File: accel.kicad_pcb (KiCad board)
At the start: 2 copper layers, 33 x 58 mm, 3 parts, among them U1 CH376T, U2 MPU-6050

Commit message: updates
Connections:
- A1 pad 7: unconnected-(A1-Pad7) -> Net-(A1-Pad7)
- U1 pad 13: unconnected-(U1-Pad13) -> Net-(A1-Pad7)

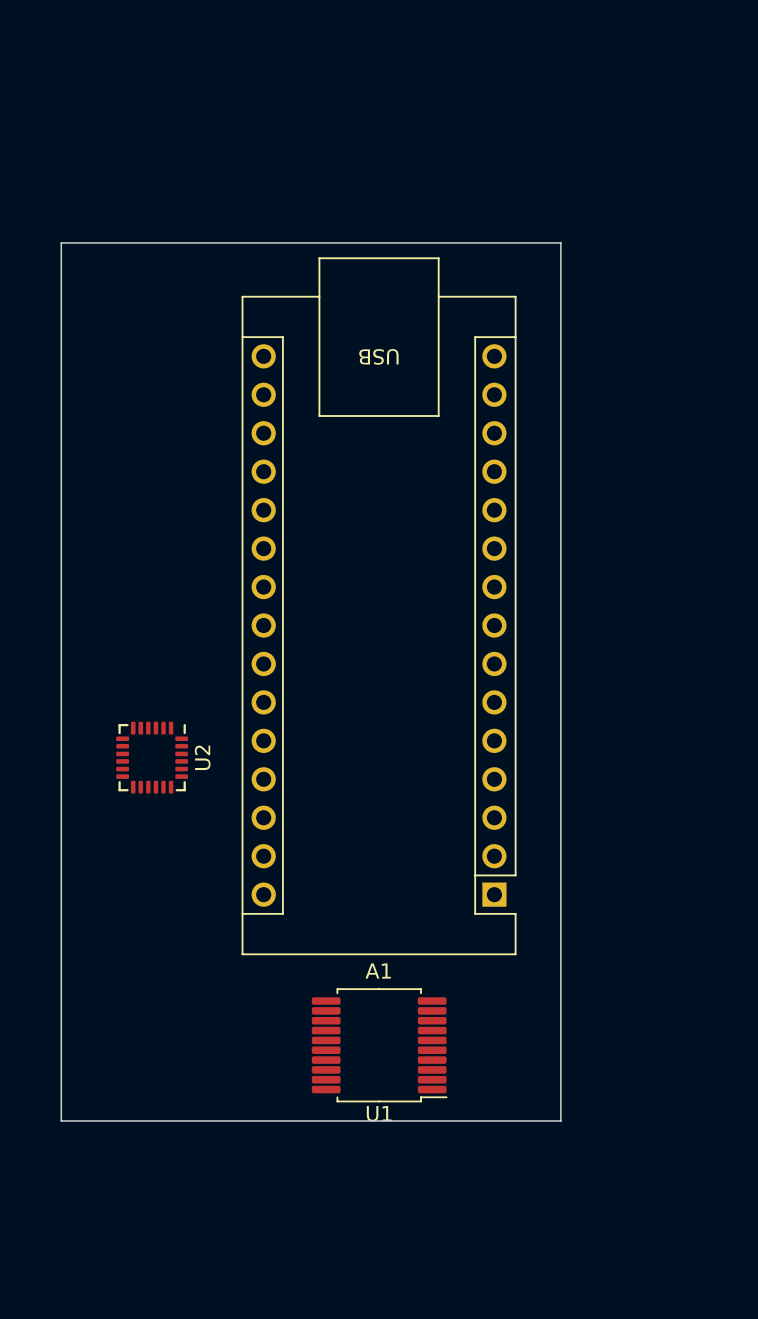
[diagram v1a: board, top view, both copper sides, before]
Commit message: final .ino and cad updates
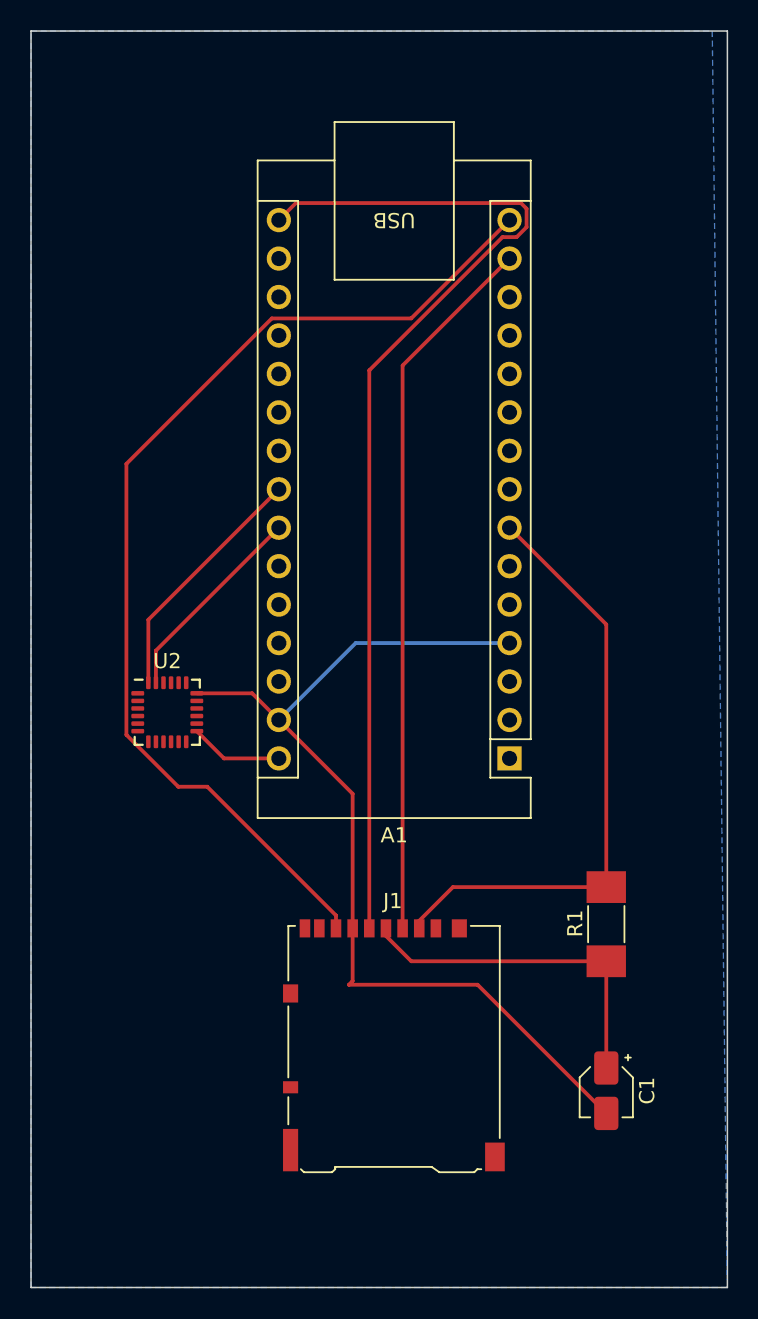
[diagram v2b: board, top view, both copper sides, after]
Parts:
- removed U1: CH376T, Package_SO:SSOP-20_5.3x7.2mm_P0.65mm
- added C1: 100nF, Capacitor_SMD:CP_Elec_3x5.4, F.Cu at (169.0, 131.0)
- added J1: Micro_SD_Card, Connector_Card:microSD_HC_Hirose_DM3AT-SF-PEJM5, F.Cu at (155.0, 128.0)
- added R1: 1K, Resistor_SMD:R_MELF_MMB-0207, F.Cu at (169.0, 120.0)
- moved A1 9.06 mm to (162.6, 109.0)
- moved U2 3.16 mm to (140.0, 106.0), turned to 0 degrees
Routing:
- net Net-(A1-Pad15): track 0.00 -> 69.5 mm
- net Net-(A1-Pad16): track 0.00 -> 69.4 mm
- net GND: track 0.00 -> 63.6 mm
- net Net-(A1-Pad14): track 0.00 -> 47.2 mm
- net Net-(A1-Pad7): track 0.00 -> 40.2 mm
- net +3V3: track 0.00 -> 22.8 mm
- net Net-(A1-Pad23): track 0.00 -> 16.4 mm
- net Net-(A1-Pad24): track 0.00 -> 13.6 mm
- net +5V: track 0.00 -> 6.17 mm
- added copper zone on B.Cu, net GND
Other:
- board size 33 x 58 mm -> 46 x 83 mm
